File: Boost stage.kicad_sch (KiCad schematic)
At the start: 9 parts, among them U57 INA2227AIYBJR, U64 TPL0102-100PWR

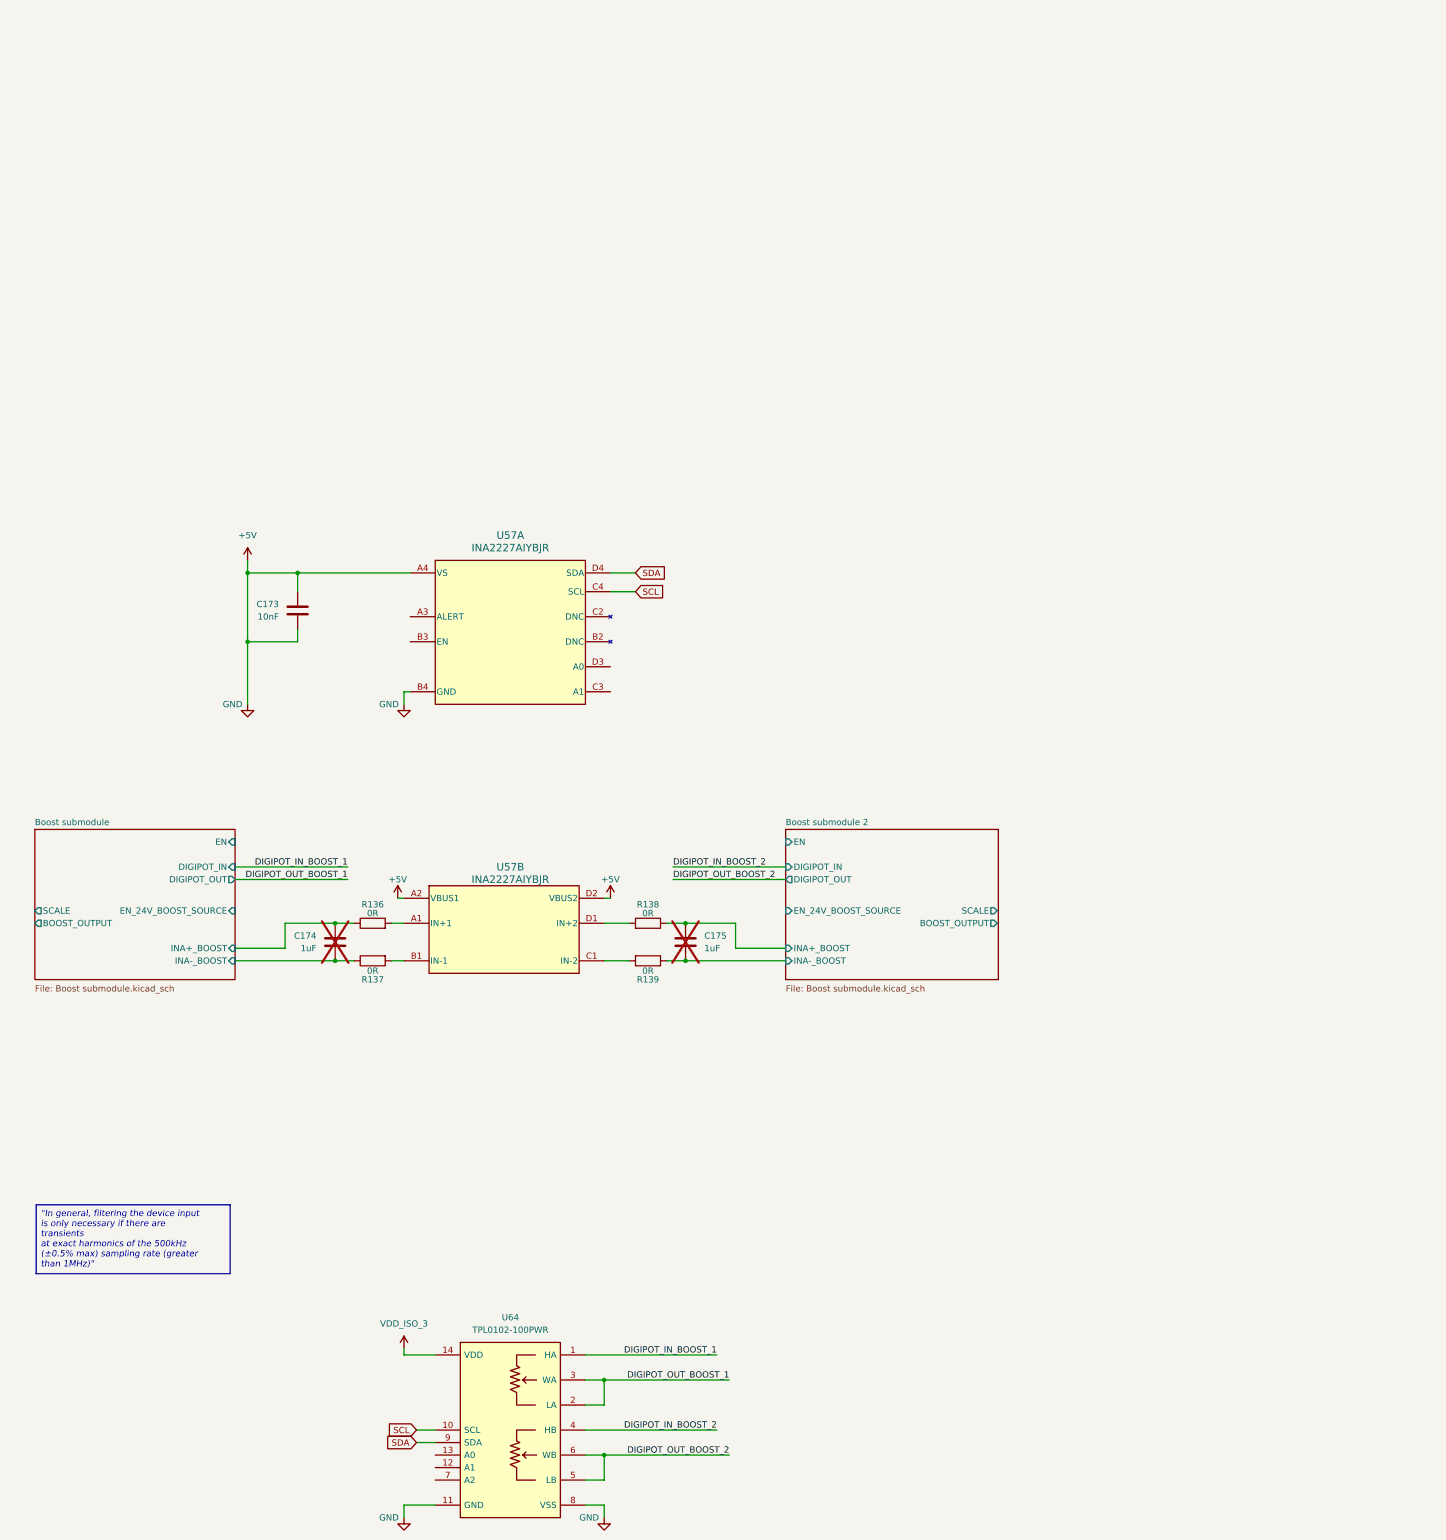
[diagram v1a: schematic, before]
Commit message: Details to finish
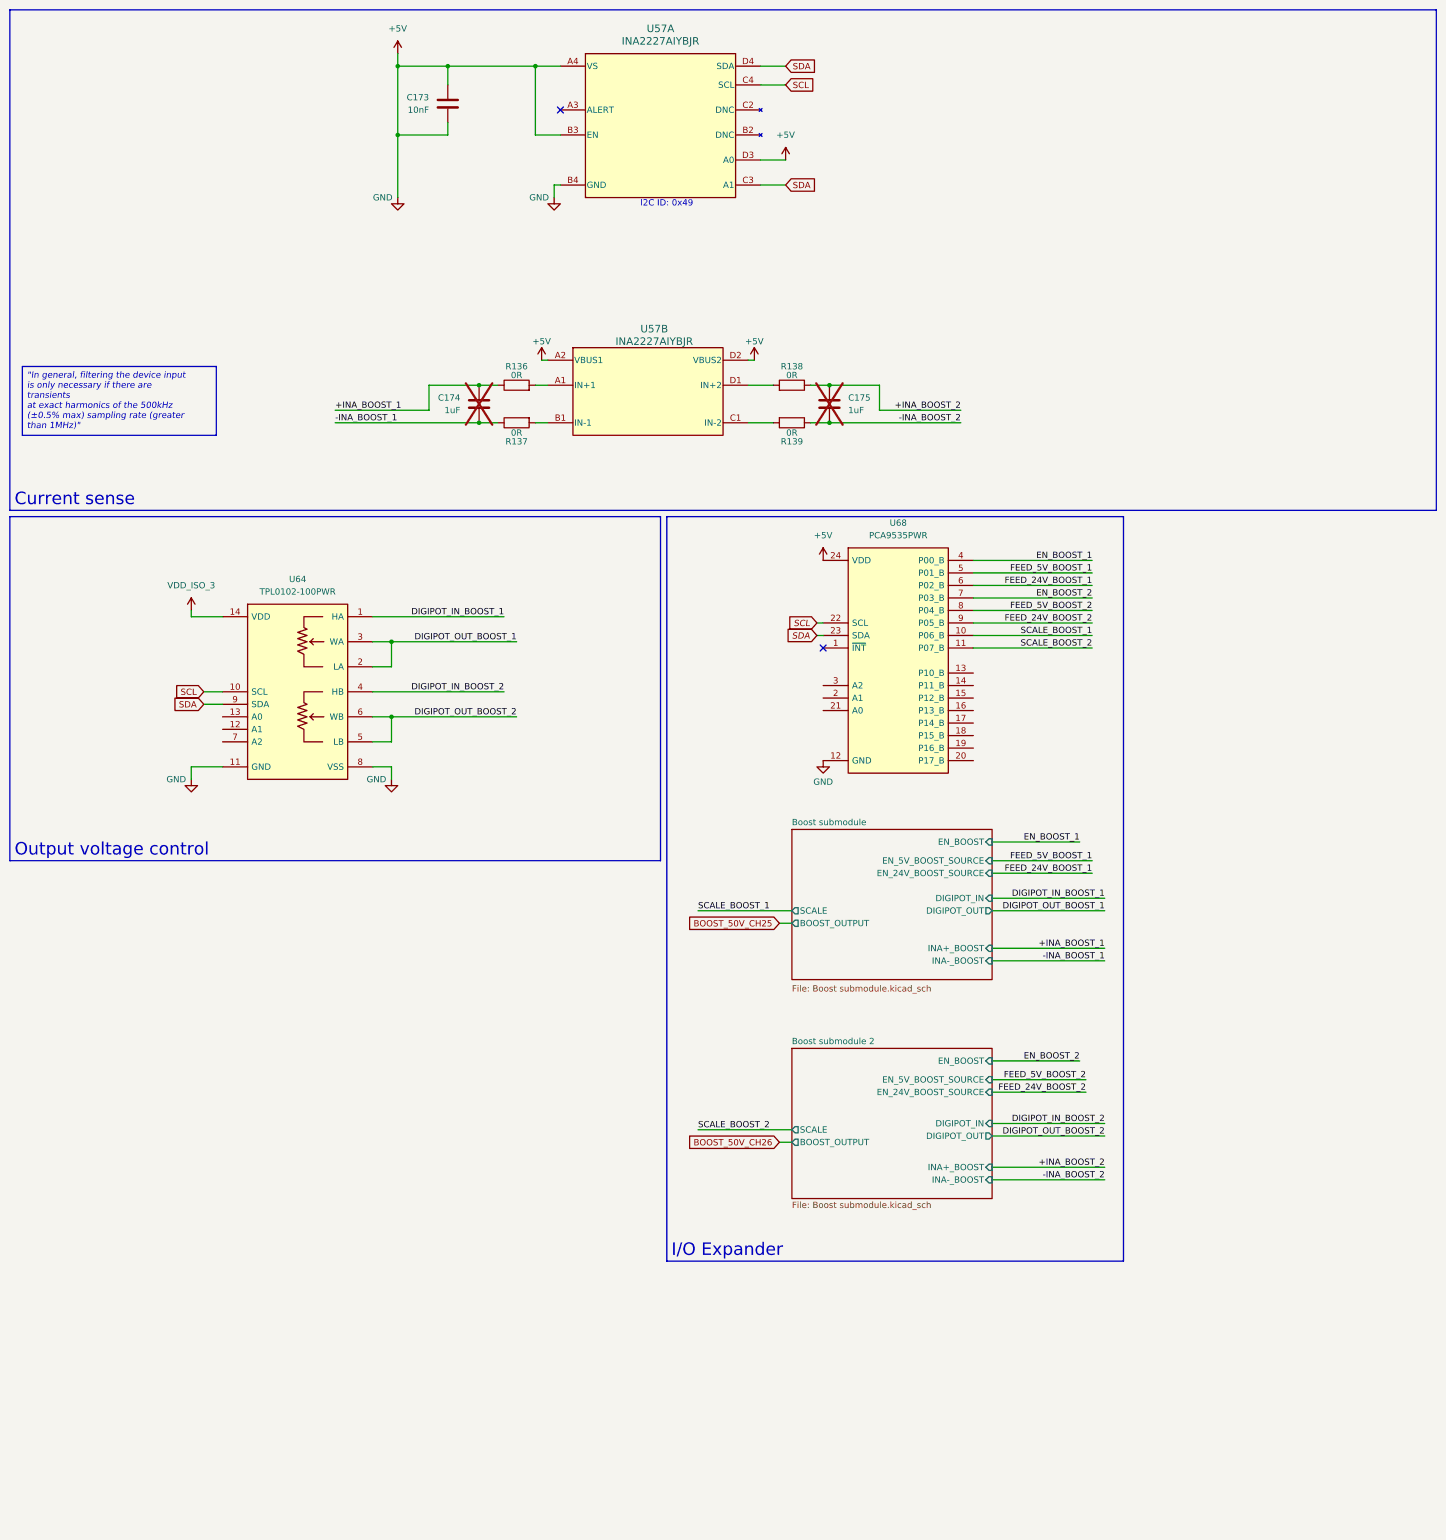
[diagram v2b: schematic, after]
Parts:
- added U68: PCA9535PWR, semiconductor:TSSOP-24_P0.65_7.8x4.4x1.2, symbol integrated-circuit:PCA9535PWR
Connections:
- net +5V: now also U57.B3 (EN), U57.D3 (A0), U68.12 (GND), U68.24 (VDD)
- net SCL: now also U68.22 (SCL)
- net SDA: now also U57.C3 (A1), U68.23 (SDA)
- net Boost submodule 2/INA+_BOOST renamed +INA_BOOST_2
- net Boost submodule 2/INA-_BOOST renamed -INA_BOOST_2
- net Boost submodule/INA+_BOOST renamed +INA_BOOST_1
- net Boost submodule/INA-_BOOST renamed -INA_BOOST_1
- new net EN_BOOST_1: U68.4 (P00_B)
- new net EN_BOOST_2: U68.7 (P03_B)
- new net FEED_24V_BOOST_1: U68.6 (P02_B)
- new net FEED_24V_BOOST_2: U68.9 (P05_B)
- new net FEED_5V_BOOST_1: U68.5 (P01_B)
- new net FEED_5V_BOOST_2: U68.8 (P04_B)
- new net SCALE_BOOST_1: U68.10 (P06_B)
- new net SCALE_BOOST_2: U68.11 (P07_B)
- no-connect marks 0 -> 2
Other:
- sheet Boost submodule ports: added EN_5V_BOOST_SOURCE, EN_BOOST; removed EN
- sheet Boost submodule 2 ports: added EN_5V_BOOST_SOURCE, EN_BOOST; removed EN
- note added: "I2C ID: 0x49"
- moved on the sheet: C173, C174, C175, R136, R137, R138, R139, U57A, U57B, U64
